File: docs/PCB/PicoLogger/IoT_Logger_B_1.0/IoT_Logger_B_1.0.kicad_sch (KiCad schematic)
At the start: 31 parts, among them J1 JTAG, U1 STM32F412RGTx, Y1 3225-25M-SR, Y2 32.768K-CFPX217

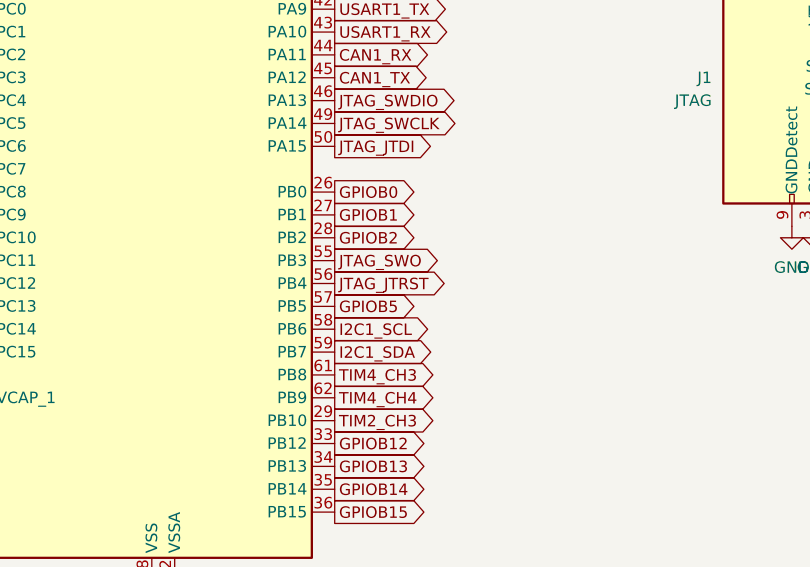
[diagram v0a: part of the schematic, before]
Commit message: Code added, documentation review.
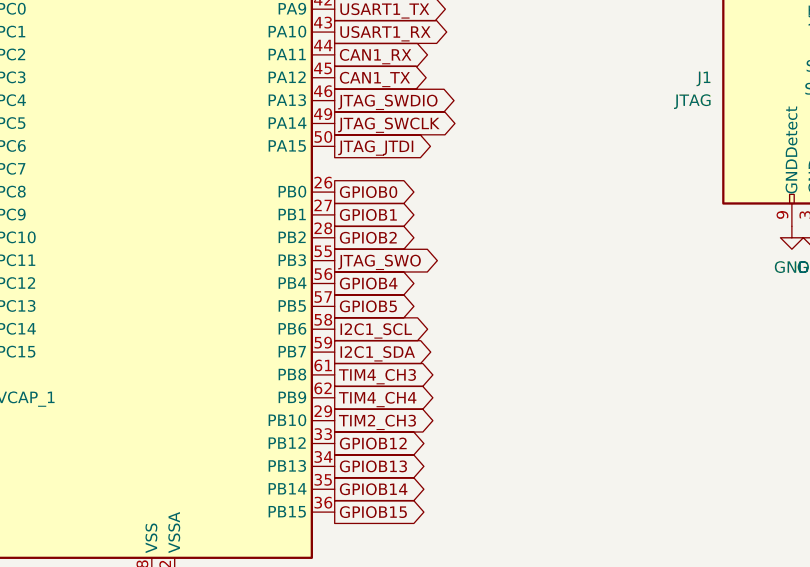
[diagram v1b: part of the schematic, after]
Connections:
- net JTAG_JTRST renamed GPIOB4
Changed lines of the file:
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@@
 		)
 	)
-	(global_label "JTAG_JTRST"
+	(global_label "GPIOB4"
 		(shape output)
 		(at 171.45 128.27 0)
@@
 		)
 		(property "Intersheetrefs" "${INTERSHEET_REFS}"
-			(at 185.0789 128.27 0)
+			(at 181.39 128.27 0)
 			(effects
 				(font
